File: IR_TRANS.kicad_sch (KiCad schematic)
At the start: 13 parts, among them Q10 XYC-PT204B-L1, U3 HT2348ARTZ8

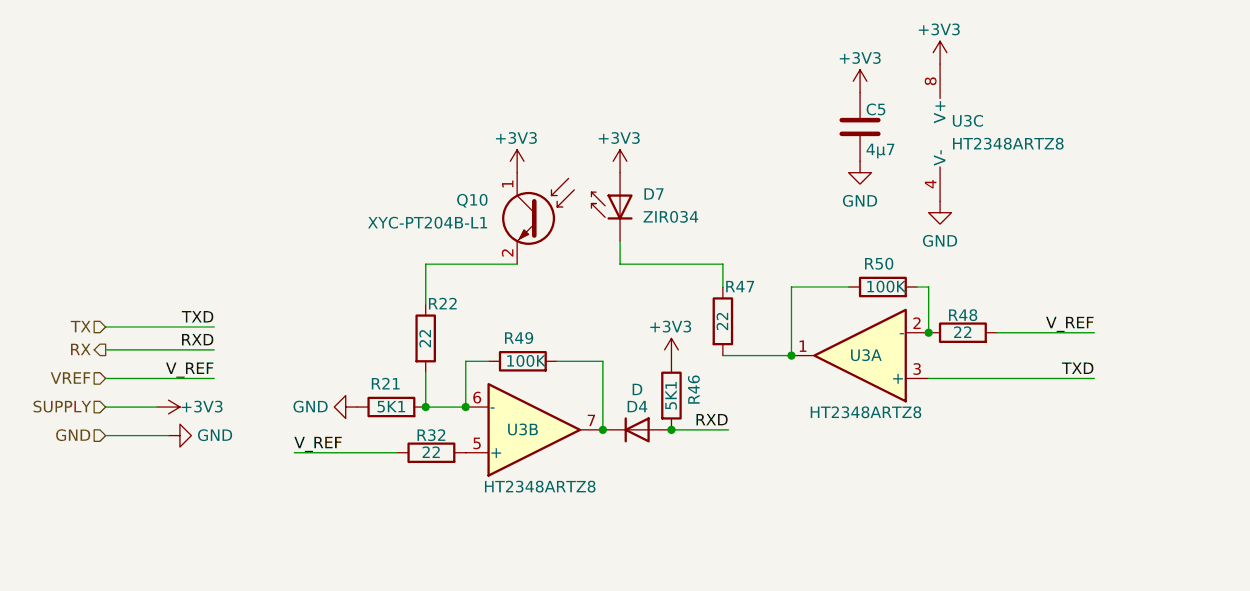
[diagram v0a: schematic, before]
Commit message: Order V1
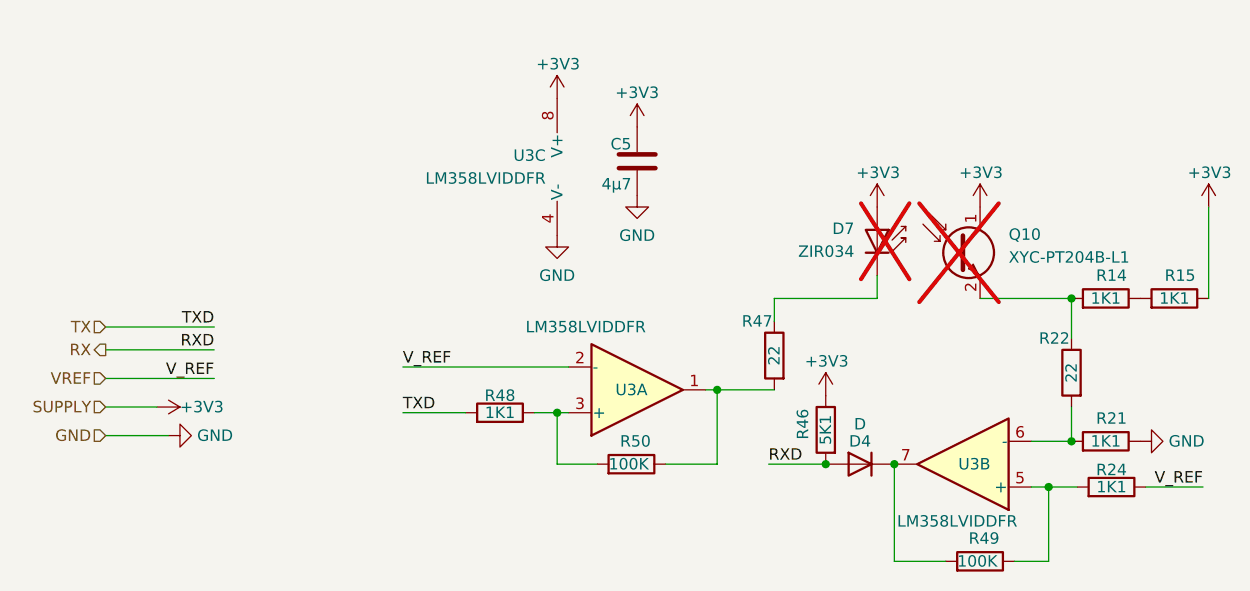
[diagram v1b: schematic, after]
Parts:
- removed R32: 22, Resistor_SMD:R_0603_1608Metric, symbol Device:R
- added R14, R15, R24: 1K1, Resistor_SMD:R_0603_1608Metric, symbol Device:R
- D7, Q10: now not fitted; now left out of the parts list
- R21: value 5K1 -> 1K1; LCSC C26000 -> C2906975
- R48: value 22 -> 1K1; LCSC C1203 -> C2906975
- U3: value HT2348ARTZ8 -> LM358LVIDDFR; LCSC C5143016 -> C1849428
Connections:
- net +3V3: now also R15.1
- net TX: now also R48.2; no longer U3.3 (+)
- net VREF: now also U3.2 (-), R24.1; no longer R48.2
- net at R48.1, R50.2: now also U3.3 (+); no longer U3.2 (-)
- net at U3.5 (+): now also R49.1, R24.2
- net at R21.2, R22.2, U3.6 (-): no longer R49.1
- net at Q10.2 (E), R22.1: now also R14.2
- new net: R14.1, R15.2
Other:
- moved on the sheet: C5, D4, R21, R22, R46, R47, R48, R49, R50, U3A, U3B, U3C
